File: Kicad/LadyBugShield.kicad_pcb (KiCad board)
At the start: 2 copper layers, 81.3 x 53.3 mm, 55 parts, among them P1 CONN_6, P2 CONN_2, P3 BNC, P4 BNC, Q1 TIP122, Q2 TIP122, Q3 TIP122, U1 MCP6244, U2 MCP6242, U3 MC78L05, U4 ADS1015

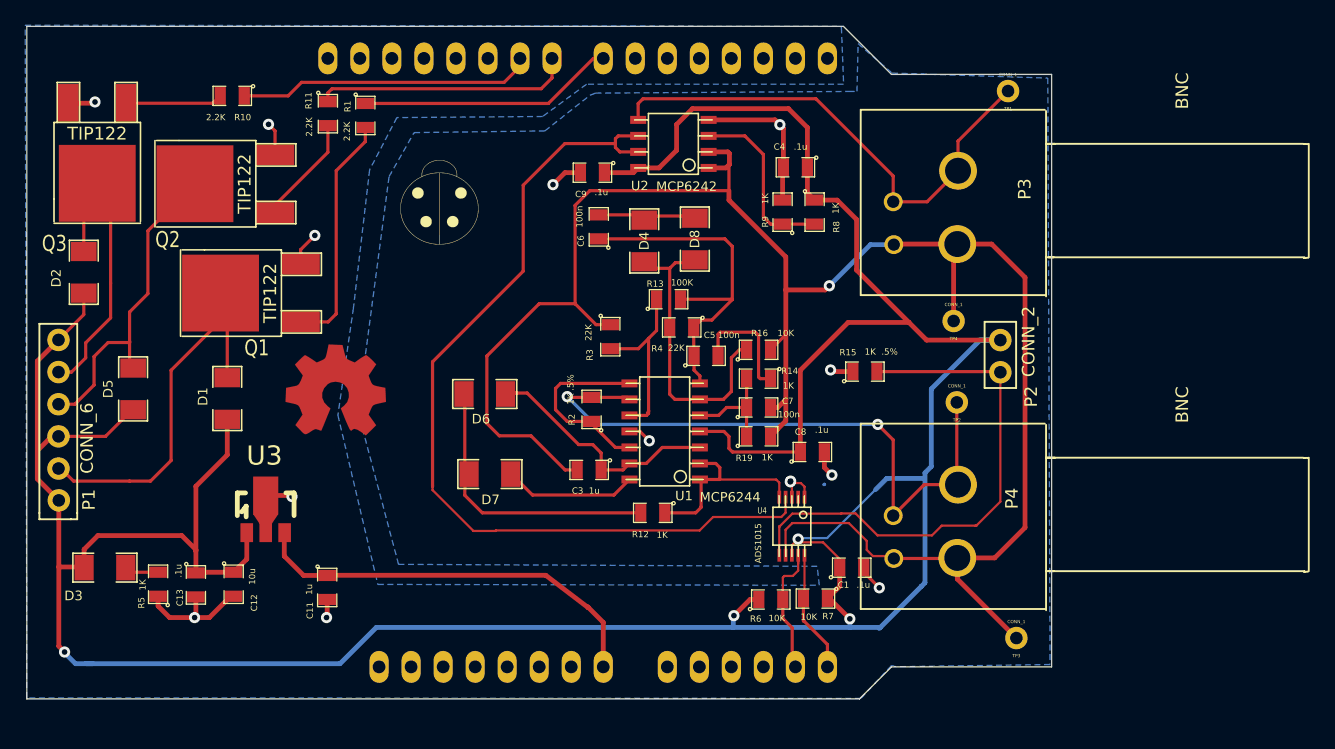
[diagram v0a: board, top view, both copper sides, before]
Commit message: changes to layout after 12/22/2014 helpout
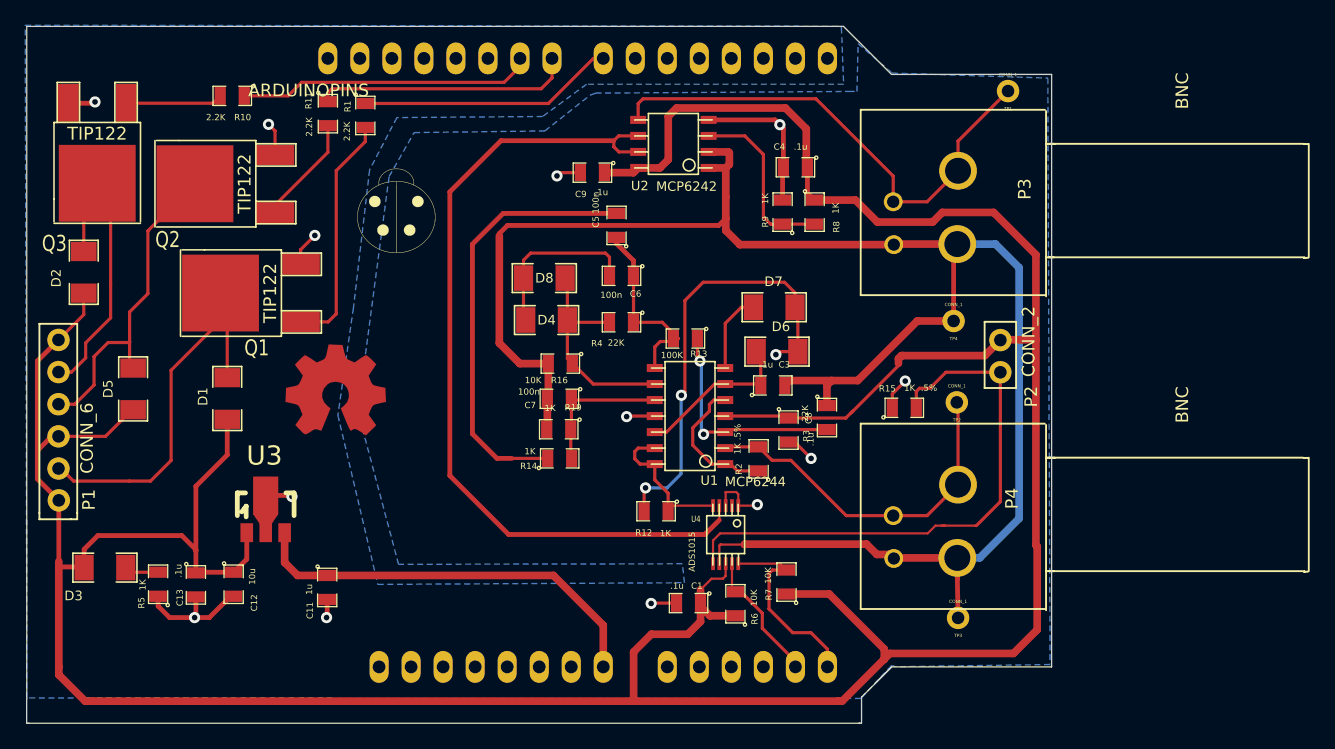
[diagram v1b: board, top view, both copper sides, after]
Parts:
- ARD1: value ~ -> ARDUINOPINS
- D1: value ~ -> 4004
- D5: value (none) -> 4004
- D6: value (none) -> DIODE
- D7: value ~ -> DIODE
- moved D7 26.1 mm to (216.8, 85.8), turned to 0 degrees
- moved D6 23.4 mm to (217.0, 89.3), turned to 180 degrees
- moved R3 18.3 mm to (220.9, 94.5)
- moved R14 17.0 mm to (199.7, 97.8), turned to 0 degrees
- moved C3 16.0 mm to (216.6, 92.0), turned to 0 degrees
- moved R19 15.9 mm to (199.7, 95.5), turned to 180 degrees
- moved C7 15.8 mm to (199.7, 93.0), turned to 180 degrees
- moved R16 15.8 mm to (199.8, 90.2), turned to 180 degrees
- moved R2 13.8 mm to (215.5, 97.8)
- moved C1 13.2 mm to (210.0, 109.2), turned to 180 degrees
- moved C5 12.5 mm to (204.3, 79.3), turned to 90 degrees
- moved D8 12.3 mm to (198.5, 83.5), turned to 180 degrees
- moved D4 9.97 mm to (198.7, 86.8), turned to 0 degrees
- moved U4 5.30 mm to (212.9, 103.8)
- moved TP3 4.89 mm to (231.3, 110.4)
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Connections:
- U1 pad 1: /DigitalAccess/EC_AIN -> EC_Signal
- U1 pad 10: AC_Shrunk -> /EC/W_Vin+
- U1 pad 12: EC_Signal -> /EC/RVin-
- U1 pad 13: /EC/RVin- -> /DigitalAccess/EC_AIN
- U1 pad 14: /EC/R_Vout -> /DigitalAccess/EC_AIN
- U1 pad 2: /DigitalAccess/EC_AIN -> /EC/EC_ProbeIN
- U1 pad 3: /EC/RVin- -> AC_Shrunk
- U1 pad 5: /EC/W_Vin+ -> EC_Signal
- U1 pad 6: /EC/W_Vin- -> /EC/RVin-
- U1 pad 7: /EC/W_Vout -> /EC/R_Vout
- U1 pad 8: EC_Signal -> /EC/W_Vout
- U1 pad 9: /EC/EC_ProbeIN -> /EC/W_Vin-
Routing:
- net /EC/f1: track 9.40 -> 34.4 mm
- net /EC/EC_ProbeIN: track 51.0 -> 28.6 mm, vias 2 -> 0
- net VClean: track 270.8 -> 290.3 mm, vias 4 -> 1
- net /EC/W_Vout: track 27.8 -> 15.2 mm
- net /EC/DD: track 22.8 -> 35.3 mm, vias 0 -> 3
- net VGND: track 157.9 -> 146.5 mm, vias 1 -> 0
- net /EC/RVin-: track 19.9 -> 12.9 mm
- net /EC/W_Vin-: track 24.2 -> 17.6 mm
- net /Arduino/SCL: track 9.72 -> 15.7 mm
- net /EC/G1: track 7.62 -> 13.5 mm
- net /DigitalAccess/pH_AIN: track 71.6 -> 66.8 mm
- net /EC/R_Vout: track 10.4 -> 6.30 mm
- net EC_Signal: track 14.9 -> 11.2 mm
- net /DigitalAccess/EC_AIN: track 15.5 -> 12.0 mm
- net AC_Shrunk: track 14.5 -> 17.7 mm, vias 0 -> 2
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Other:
- board size 81.3 x 53.3 mm -> 81.3 x 55.3 mm
- net class VClean added: clearance 0.254, trace_width 0.6096, via_dia 0.889, via_drill 0.635
